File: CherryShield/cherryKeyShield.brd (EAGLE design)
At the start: 100 x 80 mm, 19 parts

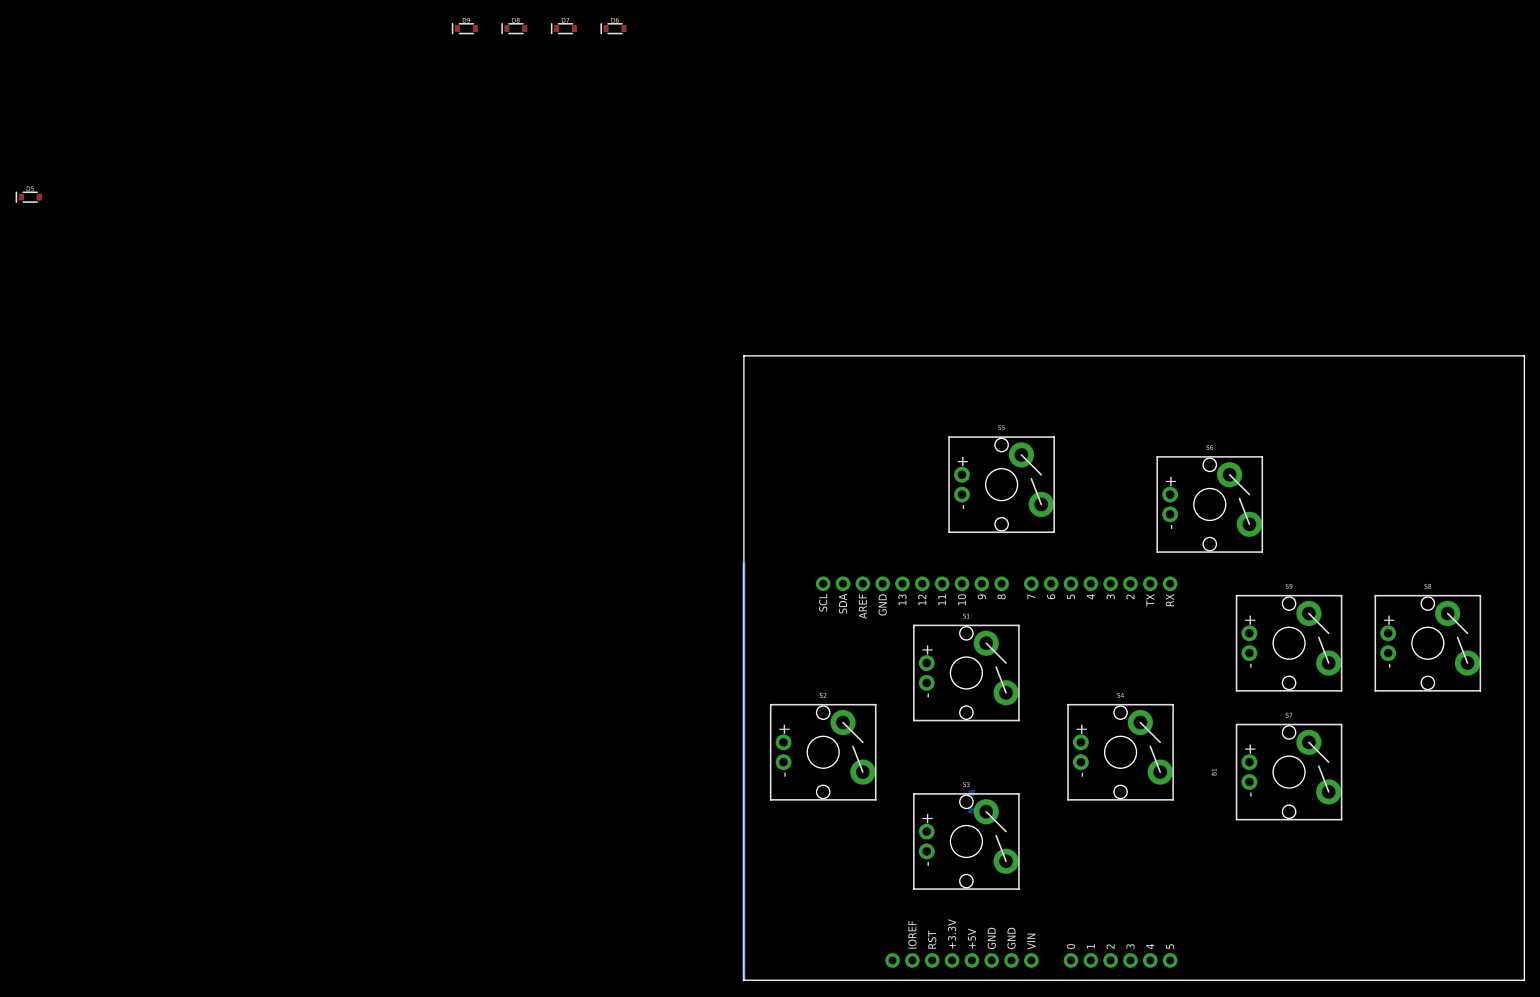
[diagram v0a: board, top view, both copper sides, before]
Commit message: newer layout
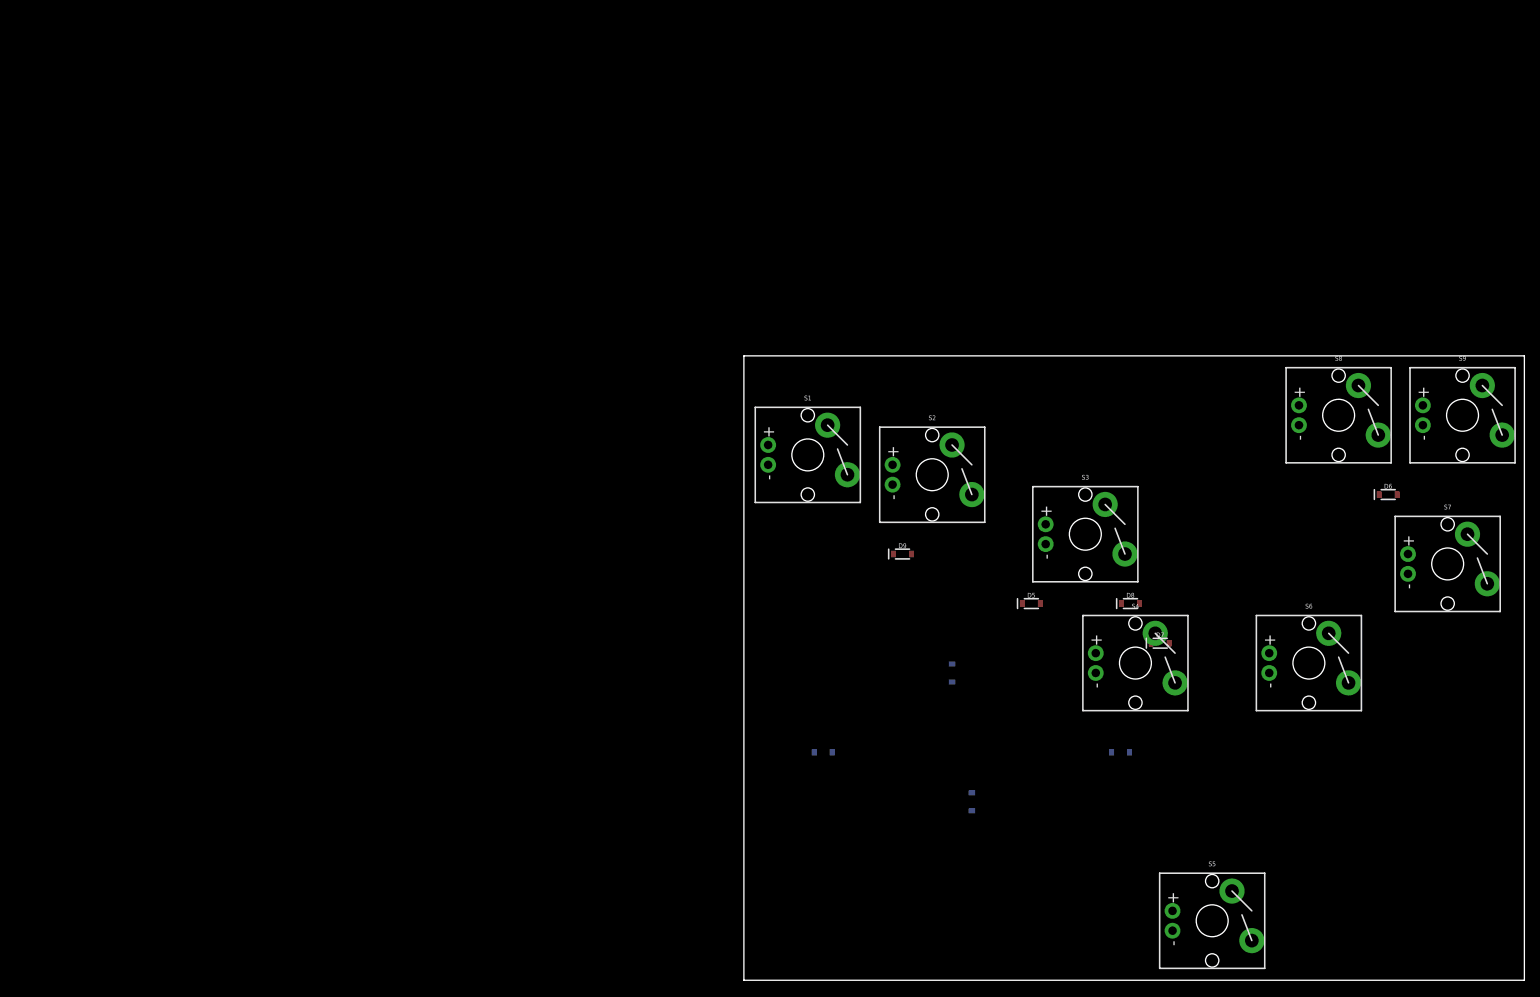
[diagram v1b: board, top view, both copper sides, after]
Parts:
- removed B1: ARDUINO_UNO_R3_SHIELDBASIC, SparkFun-Boards:UNO_R3_SHIELD
- moved D5 138.4 mm to (36.8, 48.3)
- moved D6 115.7 mm to (82.5, 62.2)
- moved D7 109.6 mm to (53.3, 43.2)
- moved D8 107.8 mm to (49.5, 48.3)
- moved D9 87.5 mm to (20.3, 54.6)
- moved S5 62.1 mm to (60.0, 7.62)
- moved S3 42.2 mm to (43.7, 57.1)
- moved S2 38.2 mm to (24.1, 64.8)
- moved S9 36.7 mm to (92.1, 72.4)
- moved S1 34.5 mm to (8.19, 67.3)
- moved S7 33.5 mm to (90.2, 53.3)
- moved S8 31.4 mm to (76.2, 72.4)
- moved S6 24.0 mm to (72.4, 40.6)
- moved S4 11.6 mm to (50.2, 40.6)
- moved D1 2.54 mm to (26.7, 39.4)
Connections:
- net X0: no longer B1.D11
- net X1: no longer B1.D12
- net X2: no longer B1.D13
- net Y0: no longer B1.D8
- net Y1: no longer B1.D9
- net Y2: no longer B1.D10
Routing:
- net N$3: track 53.3 -> 0.00 mm
